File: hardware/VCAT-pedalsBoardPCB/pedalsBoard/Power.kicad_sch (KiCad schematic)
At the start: 3 parts

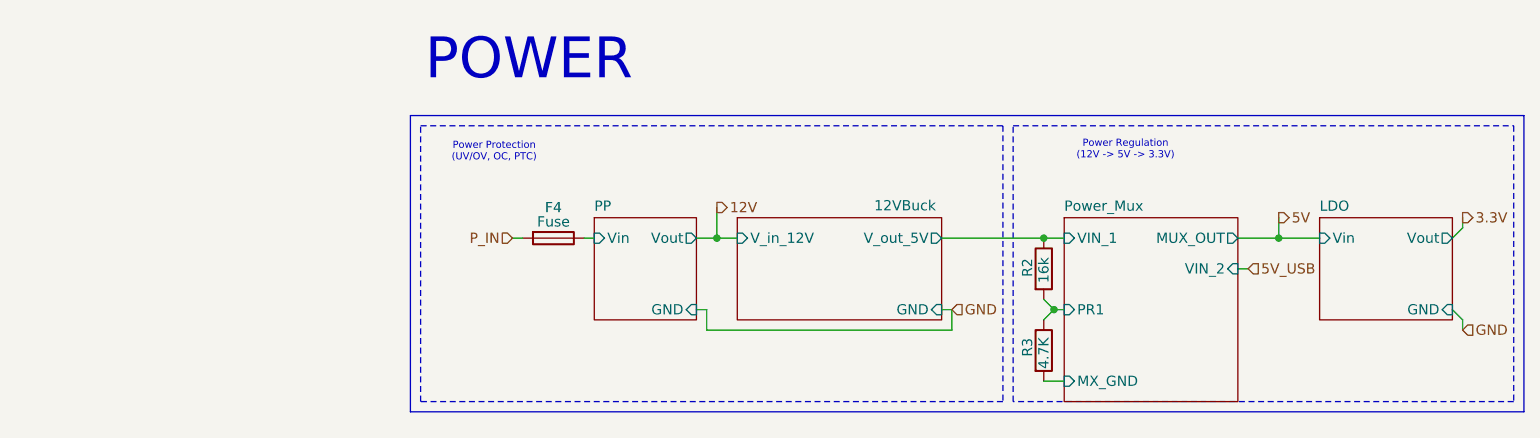
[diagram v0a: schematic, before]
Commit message: test
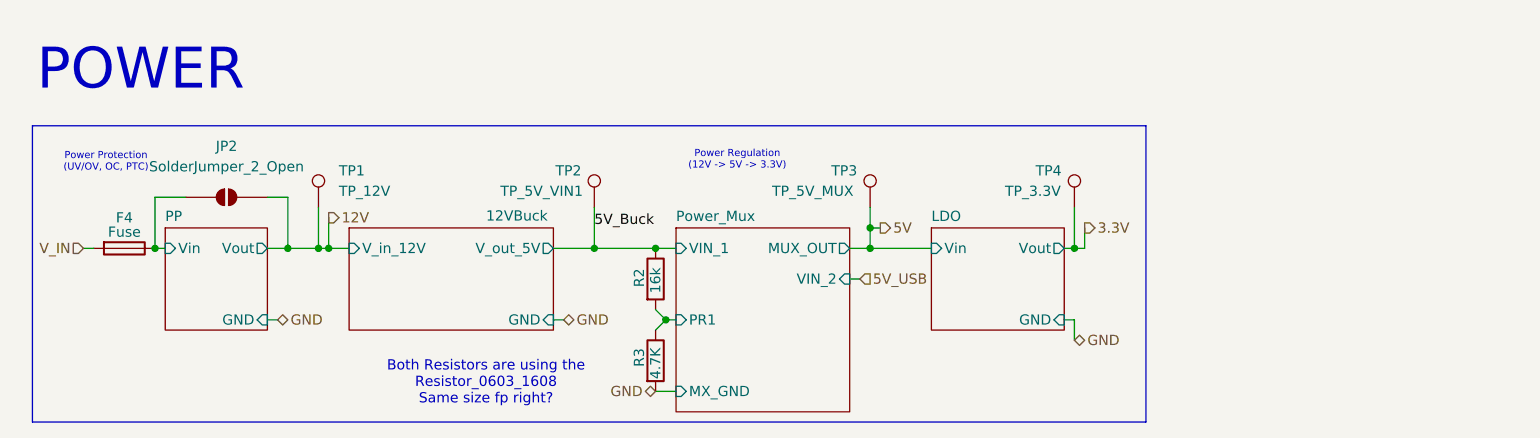
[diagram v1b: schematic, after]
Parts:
- added JP2: SolderJumper_2_Open, symbol Jumper:SolderJumper_2_Open
- added TP1: TP_12V, symbol Connector:TestPoint
- added TP2: TP_5V_VIN1, symbol Connector:TestPoint
- added TP3: TP_5V_MUX, symbol Connector:TestPoint
- added TP4: TP_3.3V, symbol Connector:TestPoint
- F4: footprint 3557-2 -> MyParts:3557-2
- R2, R3: footprint (none) -> Resistor_SMD:R_0603_1608Metric
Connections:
- net Power_Mux/MX_GND is gone; now on net GND: R3.2
- net 12V: now also JP2.2 (B), TP1.1
- net 3.3V: now also TP4.1
- net 5V: now also TP3.1
- net PP/Vin: now also JP2.1 (A)
- net 12VBuck/V_out_5V renamed 5V_Buck
- net 5V_Buck: now also TP2.1
- net P_IN renamed V_IN
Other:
- note added: "Both Resistors are using the Resistor_0603_1608 Same size fp right?"
- moved on the sheet: F4, R2, R3
